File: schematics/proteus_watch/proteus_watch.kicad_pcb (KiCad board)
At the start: 4 copper layers, 81.9 x 48.3 mm, 178 parts, among them J1 2167010509_MOLEX, J10 BAT+, J11 BAT-, J12 BAT+, J13 BAT-, J14 2167010509_MOLEX, J2 SOLDER PAD, J3 SOLDER PAD, J4 UJ20-C-H-G-SMT-2A-P16-TR, J5 2167010509_MOLEX, J7 2167010509_MOLEX, J8 MOTOR+, J9 MOTOR-, Q10 MMBT2222ALT3G, Q11 MMBT2222ALT3G, Q12 MMBT2222ALT3G, Q13 MMBT2222ALT3G, Q14 MMBT2222ALT3G, Q15 MMBT2222ALT3G, Q16 MMBT2222ALT3G, Q2 RE1C002UN, Q3 RE1C002UN, Q4 S8050, Q5 S8050, Q6 MMBT2222ALT3G, Q7 FS8205, Q8 FS8205, Q9 MMBT2222ALT3G, SW1 R-667995, SW2 R-667995, SW3 EVQ-P7A01P, SW4 EVQ-P7A01P, SW5 EVQ-P7A01P, U1 MAX17048G+T10, U10 LSM6DSO, U11 BQ25185, U12 NCP186AMX330TAG, U13 CP2102N-Axx-xQFN28, U14 DRV2605LDGS, U15 DW01A, U18 DW01A, U21 SN74HC595NSR, U22 SN74HC595NSR, U3 MIC2876-5.0YMT-TR, U4 MIC5365-1.8YMT-TZ, U5 NCP186AMX330TAG, U6 ESP32-S3-MINI-1, U7 MAX30101EFD_T, U8 PCF85063ATL, Y1 32.768kHZ, 7pF, 60kOhms

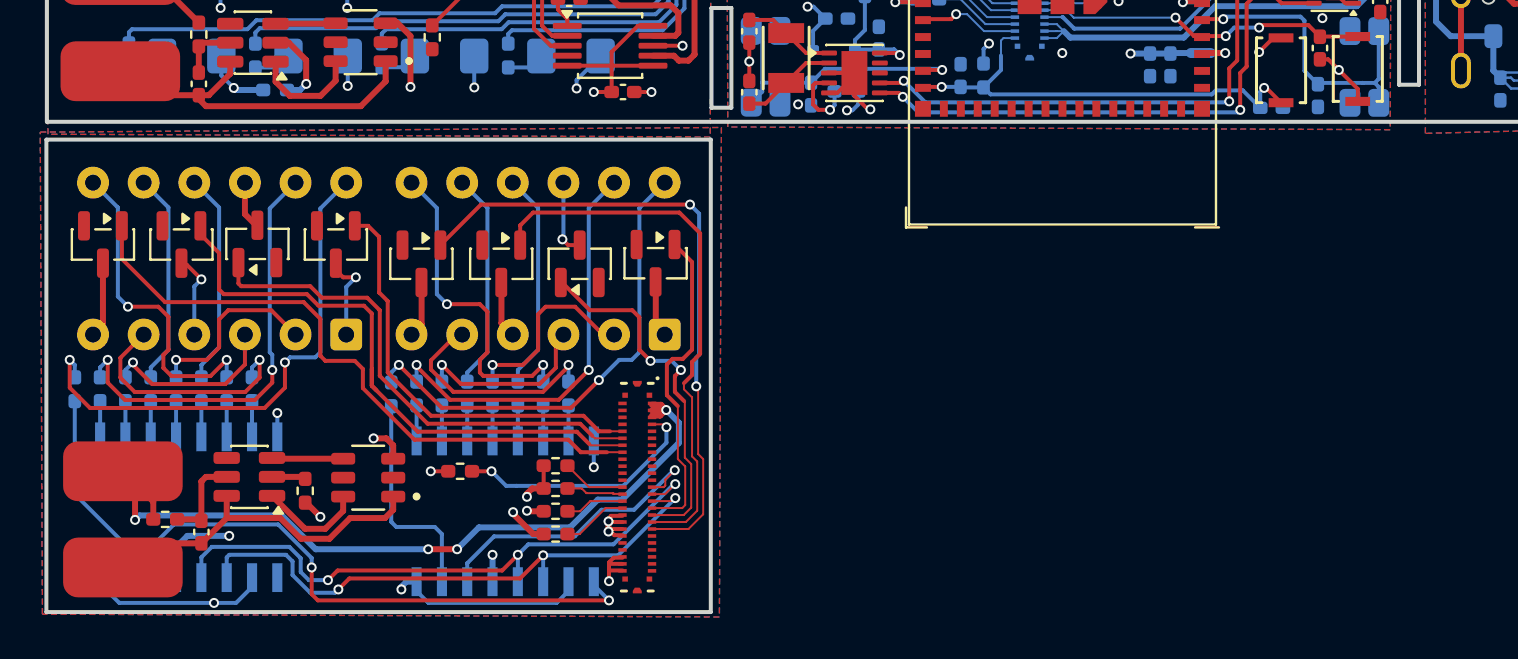
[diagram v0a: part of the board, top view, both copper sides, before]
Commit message: v1.31
wip integrating face3
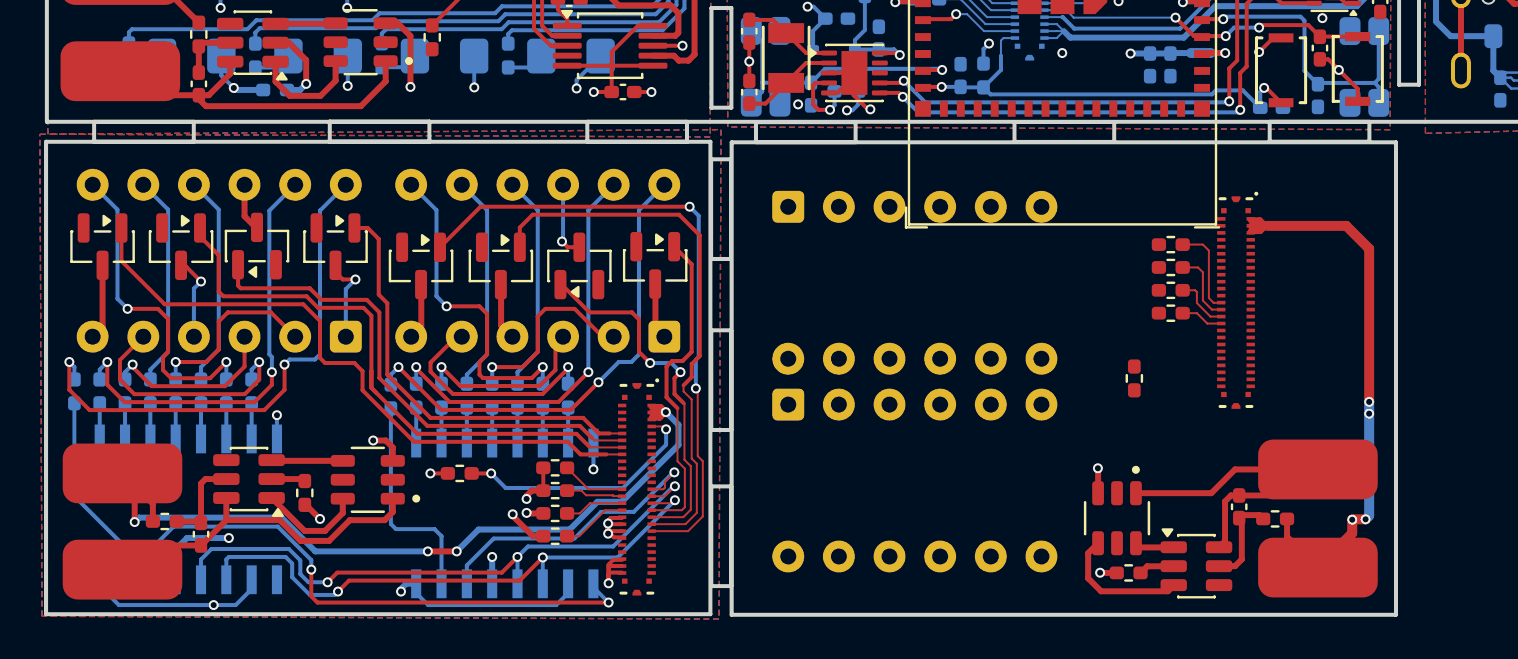
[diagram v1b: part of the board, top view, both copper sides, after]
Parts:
- added C37: 0.1uF, Capacitor_SMD:C_0402_1005Metric_Pad0.74x0.62mm_HandSolder, F.Cu at (145.2, 140.2)
- added DS1: HCMS-2901, Package_DIP:DIP-12_W7.62mm, B.Cu at (122.5, 135.1)
- added DS2: HCMS-2901, Package_DIP:DIP-12_W7.62mm, B.Cu at (122.5, 125.2)
- added J15: BAT+, Connector_Wire:SolderWirePad_1x01_SMD_3x6mm, F.Cu at (149.1, 143.3)
- added J16: BAT-, Connector_Wire:SolderWirePad_1x01_SMD_3x6mm, F.Cu at (149.1, 138.3)
- added J17: 2167010509_MOLEX, footprint:CON_2167010509_MOL, F.Cu at (145.0, 130.0)
- added Q17: FS8205, footprint:SOT95P280X145-6N, F.Cu at (139.0, 140.8)
- added R73: 100, Resistor_SMD:R_0402_1005Metric_Pad0.72x0.64mm_HandSolder, F.Cu at (147.0, 140.8)
- added R74: 10K, Resistor_SMD:R_0402_1005Metric_Pad0.72x0.64mm_HandSolder, F.Cu at (141.7, 127.1)
- added R75: 10K, Resistor_SMD:R_0402_1005Metric_Pad0.72x0.64mm_HandSolder, F.Cu at (141.7, 128.2)
- added R76: 10K, Resistor_SMD:R_0402_1005Metric_Pad0.72x0.64mm_HandSolder, F.Cu at (141.7, 129.4)
- added R77: 10K, Resistor_SMD:R_0402_1005Metric_Pad0.72x0.64mm_HandSolder, F.Cu at (141.7, 130.5)
- added R78: 1K, Resistor_SMD:R_0402_1005Metric_Pad0.72x0.64mm_HandSolder, F.Cu at (139.6, 143.5)
- added TH3: 10K, Resistor_SMD:R_0402_1005Metric_Pad0.72x0.64mm_HandSolder, F.Cu at (139.9, 133.8)
- added U23: DW01A, Package_TO_SOT_SMD:SOT-23-6, F.Cu at (143.0, 143.2)
- moved Q10 0.11 mm to (112.1, 128.1)
- moved Q11 0.11 mm to (108.1, 128.1)
- moved Q12 0.11 mm to (104.1, 128.1)
- moved Q14 0.11 mm to (95.9, 127.1)
- moved Q16 0.11 mm to (88.1, 127.2)
- moved Q8 0.11 mm to (101.4, 138.9)
- moved R52 0.11 mm to (98.3, 139.5)
- moved R57 0.11 mm to (102.6, 134.7)
- moved R59 0.11 mm to (105.1, 134.6)
- moved R60 0.11 mm to (106.4, 134.6)
- moved R61 0.11 mm to (107.7, 134.6)
- moved R63 0.11 mm to (110.2, 134.6)
- moved R64 0.11 mm to (111.5, 134.6)
- moved R65 0.11 mm to (86.7, 134.4)
- moved R67 0.11 mm to (89.3, 134.4)
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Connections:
- net Net-(J7-Pin_38) renamed /face1/GPIO48
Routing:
- net /face3/BAT+: track 0.00 -> 28.7 mm, vias 0 -> 4
- net Net-(J16-Pin_1): track 0.00 -> 17.4 mm
- net Net-(U23-OC): track 0.00 -> 6.67 mm
- net Net-(U23-VCC): track 0.00 -> 4.89 mm
- net /face3/GPIO48: track 0.00 -> 4.54 mm
- net /face3/GPIO34: track 0.00 -> 3.64 mm
- net /face3/GPIO33: track 0.00 -> 2.80 mm
- net /face3/GPIO47: track 0.00 -> 2.15 mm
- net F3_GND: track 0.00 -> 2.09 mm, vias 0 -> 2
- net Net-(U23-OD): track 0.00 -> 1.99 mm
- net Net-(U23-CS): track 0.00 -> 1.81 mm
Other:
- board size 81.9 x 48.3 mm -> 81.9 x 48.4 mm

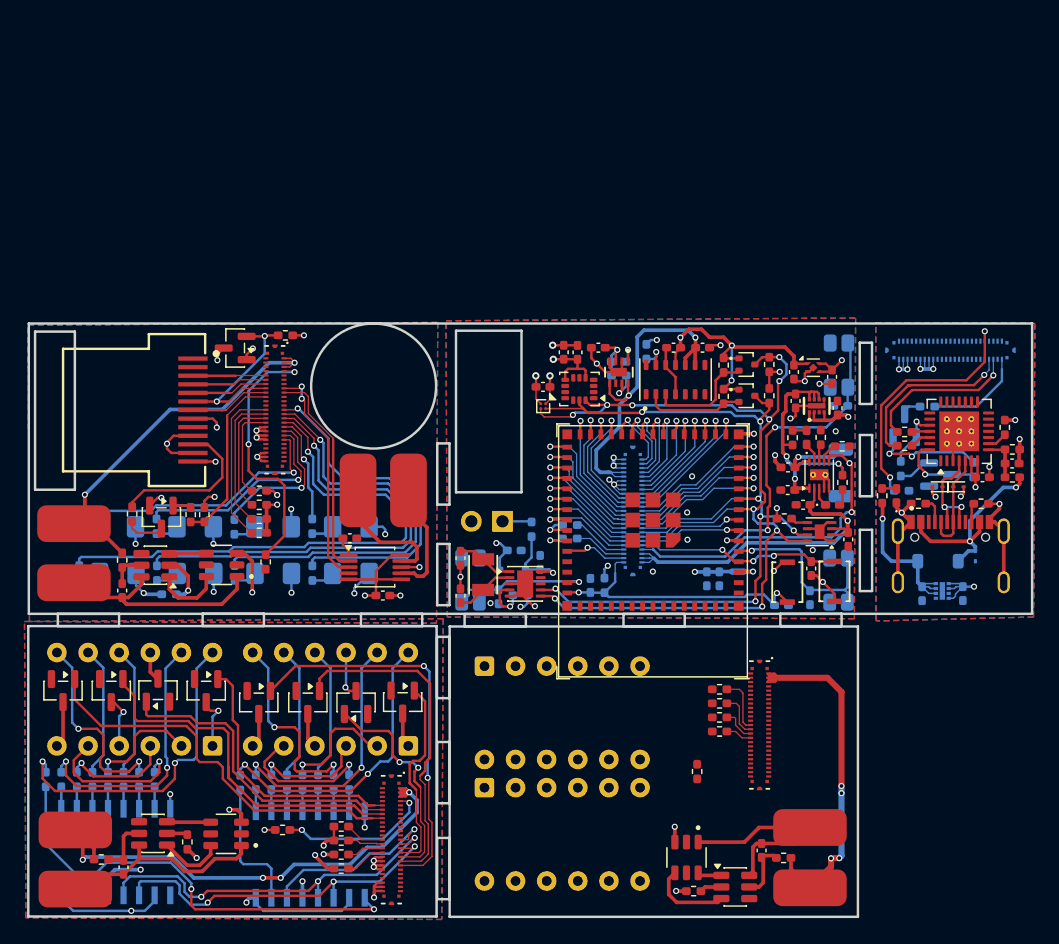
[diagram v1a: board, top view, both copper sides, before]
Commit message: v1.4
completed board layout for production
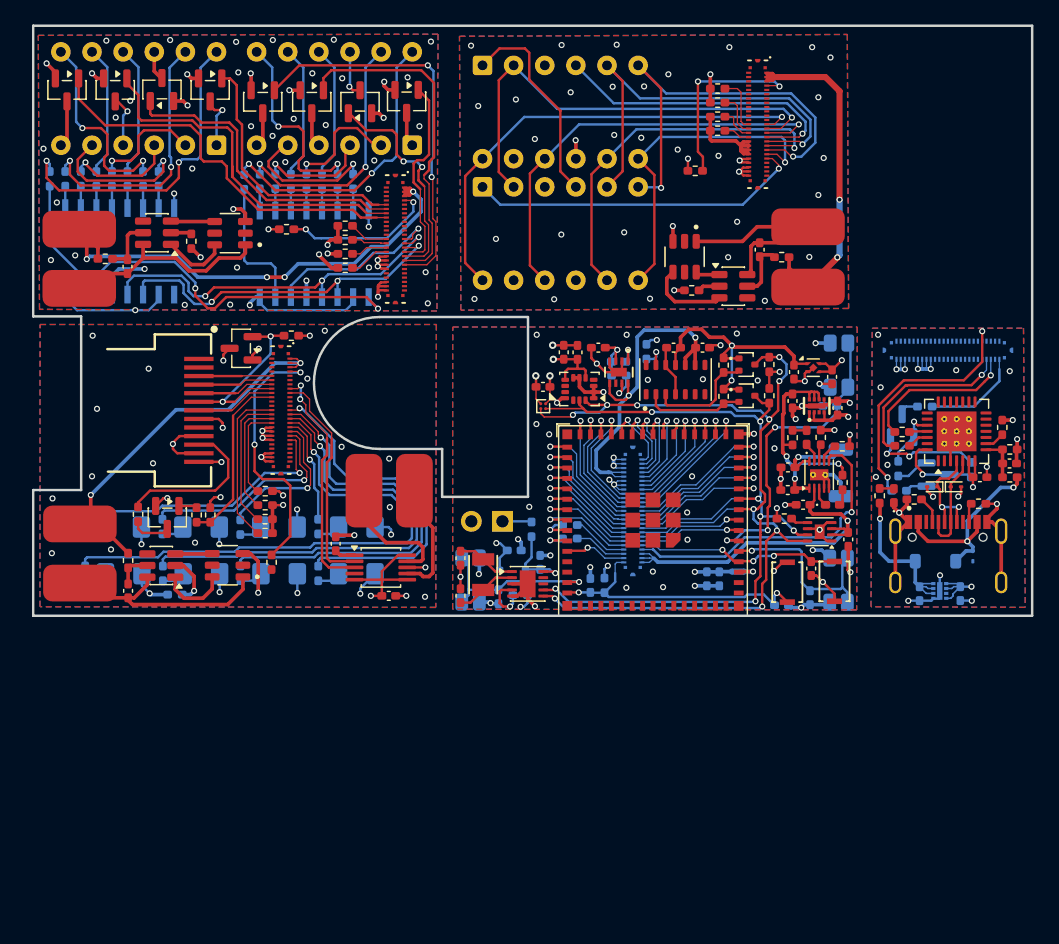
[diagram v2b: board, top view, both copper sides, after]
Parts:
- moved C37 49.0 mm to (145.0, 91.2)
- moved DS1 49.0 mm to (122.4, 86.1)
- moved DS2 49.0 mm to (122.4, 76.1)
- moved R75 49.0 mm to (141.6, 79.2)
- moved TH3 49.0 mm to (139.7, 84.7), turned to 180 degrees
- moved J15 49.0 mm to (148.9, 94.2)
- moved J16 49.0 mm to (148.9, 89.3)
- moved J17 49.0 mm to (144.8, 80.9)
- moved Q17 49.0 mm to (138.9, 91.8)
- moved R73 49.0 mm to (146.8, 91.8)
- moved R74 49.0 mm to (141.6, 78.0)
- moved R76 49.0 mm to (141.6, 80.3)
- moved R77 49.0 mm to (141.6, 81.5)
- moved R78 49.0 mm to (139.4, 94.5)
- moved U23 49.0 mm to (142.8, 94.2)
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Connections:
- TH3 pad 2: F2_GND -> F3_GND
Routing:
- net /face3/GPIO10: track 0.00 -> 38.4 mm, vias 0 -> 1
- net /face3/GPIO11: track 0.00 -> 37.8 mm, vias 0 -> 1
- net /face3/GPIO12: track 0.00 -> 35.7 mm, vias 0 -> 1
- net /face3/CLK: track 0.00 -> 35.6 mm, vias 0 -> 2
- net /face3/GPIO14: track 0.00 -> 34.7 mm, vias 0 -> 1
- net GND: track 47.6 -> 80.4 mm, vias 22 -> 49
- net /face3/BLANK: track 0.00 -> 30.9 mm, vias 0 -> 1
- net /face3/DOUT: track 0.00 -> 27.5 mm, vias 0 -> 1
- net /face3/CE: track 0.00 -> 27.4 mm, vias 0 -> 1
- net /face3/DIN: track 0.00 -> 24.8 mm, vias 0 -> 1
- net Net-(DS1-DATA_IN): track 0.00 -> 17.1 mm
- net Net-(J17-Pin_4): track 0.00 -> 15.4 mm, vias 0 -> 2
- net F2_GND: track 20.8 -> 30.5 mm, vias 10 -> 49
- net F3_3V3: track 0.00 -> 8.01 mm
- net F3_GND: track 2.09 -> 9.56 mm, vias 2 -> 36
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- added copper zone on In2.Cu, net F3_5V
- added copper zone on B.Cu, net F3_GND
- added copper zone on F.Cu, net F3_GND
- added copper zone on In1.Cu, net F3_GND
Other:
- board size 81.9 x 48.4 mm -> 81.5 x 48.2 mm
